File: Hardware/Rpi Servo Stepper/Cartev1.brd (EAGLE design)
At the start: 100 x 80 mm, 8 parts

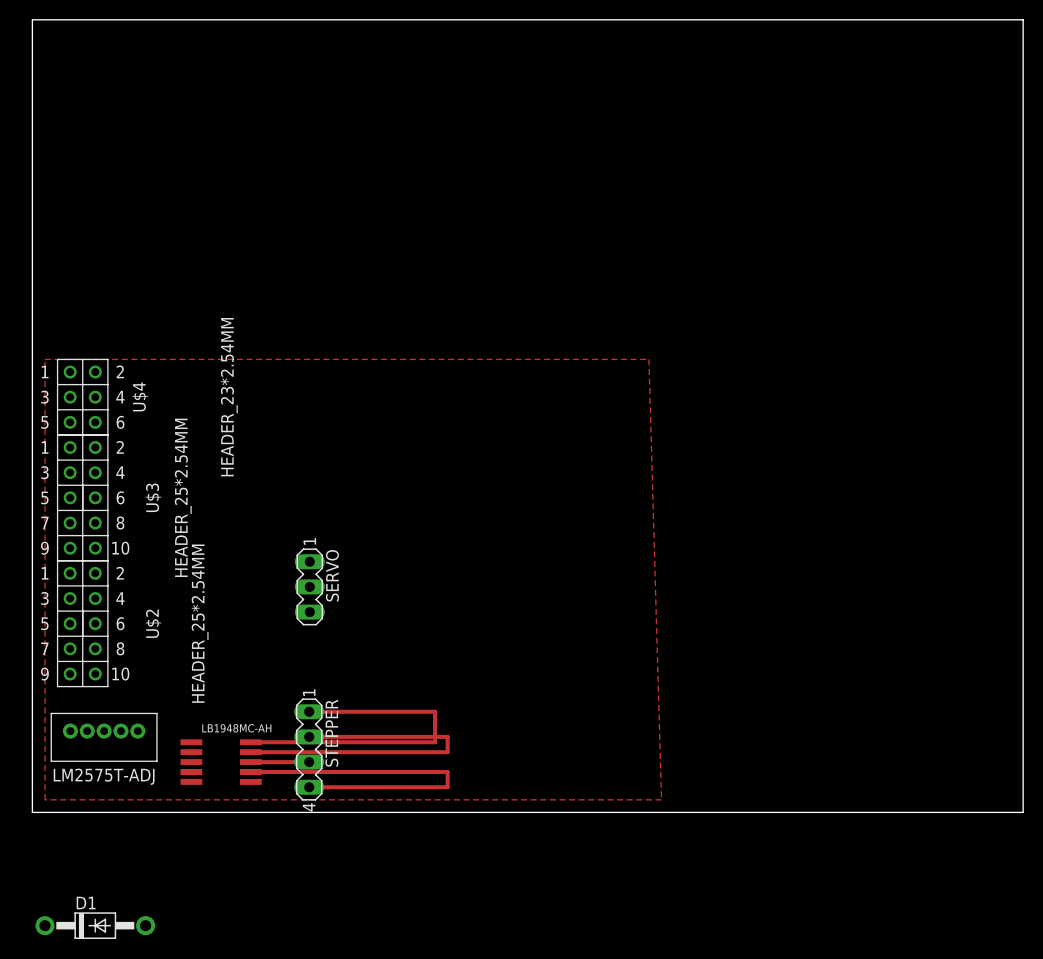
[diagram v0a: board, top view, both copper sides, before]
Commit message: Hardware V2 PROD
Version ITEAD Studio Production
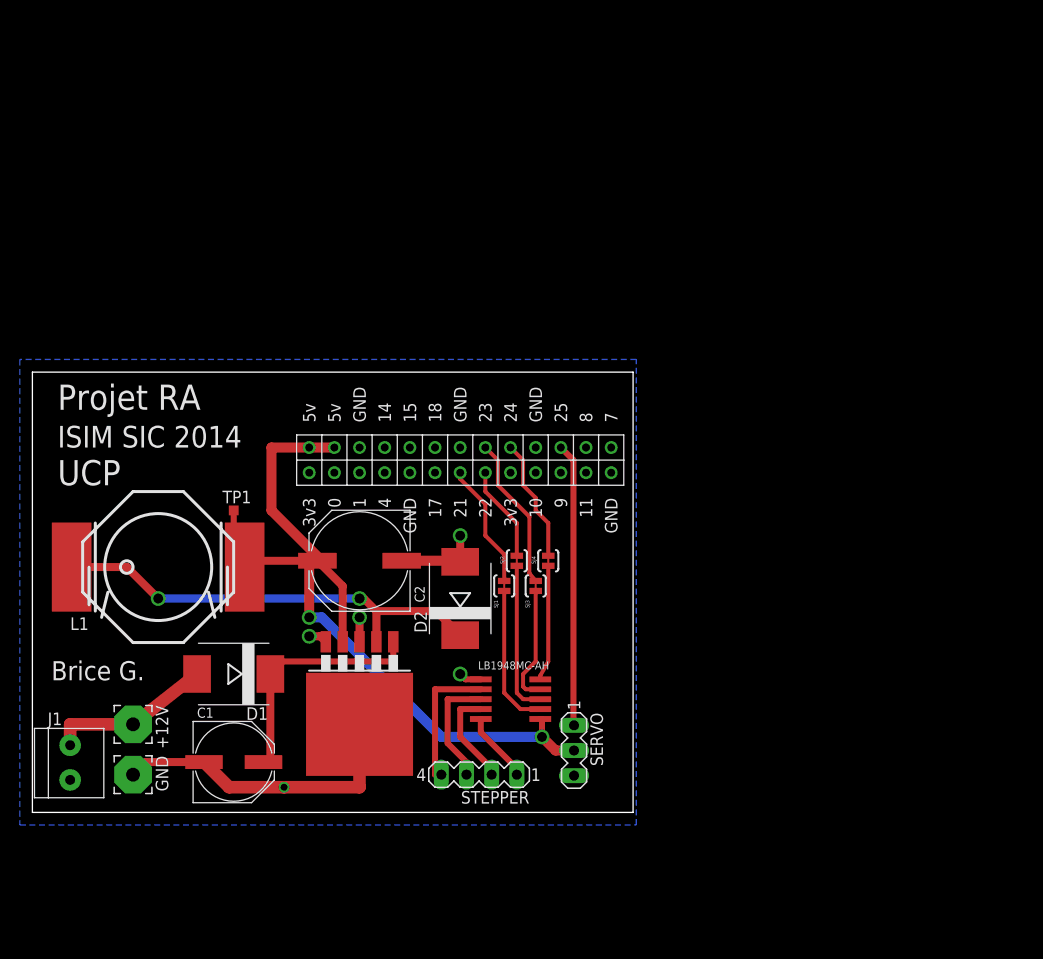
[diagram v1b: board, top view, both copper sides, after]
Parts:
- removed LM2575T-ADJ: LM2575T-ADJ, LM2575T:TO-220
- removed U$3: HEADER_25*2.54MM, Headers:2*5*2.54MM
- removed U$4: HEADER_23*2.54MM, Headers:2*3*2.54MM
- added +12V, GND: (no value), wirepad:3,81/1,4
- added C1: 100uf, rcl:PANASONIC_E
- added C2: 1000uF, rcl:PANASONIC_G
- added D2: (no value), diode:SMC
- added J1: 1X2-3.5MM, adafruit (2):3.5MMTERM
- added L1: SDR2207, bourns-inductor:SM
- added LM1: LM2576-5V, linear:TO263-5
- added SJ1, SJ2, SJ3, SJ4: (no value), SparkFun-Passives:SJ_2S-TRACE
- added TP1: TPTP10SQ, testpad:TP10SQ
- D1: value VS-11DQ06 -> (none); device adafruit:DO41-10 -> diode:SMC
- U$2: value HEADER_25*2.54MM -> CONNECTEUR_RPI; device Headers:2*5*2.54MM -> Rpi:26PIN
- moved U$2 41.5 mm to (43.2, 35.6), turned to 90 degrees
- moved SERVO 31.4 mm to (54.7, 6.25)
- moved LB1948MC-AH 29.9 mm to (48.3, 11.4), turned to 180 degrees
- moved D1 29.0 mm to (20.3, 14.0), turned to 180 degrees
- moved STEPPER 17.3 mm to (45.1, 3.81), turned to 180 degrees
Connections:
- new net +5V: C2.+, L1.P$2, LB1948MC-AH.1, LM1.4, SERVO.2, TP1.TP, U$2.5V_1, U$2.5V_2
- new net N$10: LB1948MC-AH.5, SJ4.1
- new net N$11: SERVO.1, U$2.G25
- new net N$12: SJ1.2, U$2.G21
- new net N$13: SJ2.2, U$2.G22
- new net N$14: SJ3.2, U$2.G23
- new net N$15: SJ4.2, U$2.G24
- new net N$6: D2.C, L1.P$1, LM1.2
- new net N$7: LB1948MC-AH.2, SJ1.1
- new net N$8: LB1948MC-AH.3, SJ2.1
- new net N$9: LB1948MC-AH.4, SJ3.1
- new net VDD: C1.+, D1.C, LM1.1
- net GND: now also C1.-, C2.-, D2.A, GND.1, J1.1, LM1.3, LM1.5, LM1.6, SERVO.3, U$2.GND_1, U$2.GND_2, U$2.GND_3, U$2.GND_4, U$2.GND_5; no longer LM2575T-ADJ.3
- net N$5: now also +12V.1, D1.A, J1.2; no longer LB1948MC-AH.1, LM2575T-ADJ.1
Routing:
- net +5V: track 0.00 -> 84.9 mm, vias 0 -> 2
- net GND: track 0.00 -> 49.5 mm, vias 0 -> 5
- net N$6: track 0.00 -> 45.2 mm, vias 0 -> 2
- net N$11: track 0.00 -> 28.6 mm
- net N$1: track 34.4 -> 7.13 mm
- net N$2: track 35.4 -> 10.0 mm
- net VDD: track 0.00 -> 24.6 mm
- net N$4: track 35.4 -> 13.9 mm
- net N$5: track 0.00 -> 16.7 mm
- net N$14: track 0.00 -> 15.5 mm
- net N$8: track 0.00 -> 15.5 mm
- net N$7: track 0.00 -> 14.6 mm
- net N$12: track 0.00 -> 12.8 mm
- net N$15: track 0.00 -> 12.5 mm
- net N$9: track 0.00 -> 12.0 mm
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- added copper zone on layer 16, net GND
- removed copper zone on layer 1, net GND
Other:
- board size 100 x 80 mm -> 60.6 x 44.4 mm
- board text added: "Brice G."
- board text added: "ISIM SIC 2014"
- board text added: "Projet RA"
- board text added: "UCP"
